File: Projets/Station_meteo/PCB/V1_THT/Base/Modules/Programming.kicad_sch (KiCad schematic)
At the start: 15 parts, among them J13 USB_C_Receptacle_USB2.0_16P, J14 SolderJumper_2_Bridged, J15 SolderJumper_2_Bridged, J16 SolderJumper_2_Bridged, U10 CH340G, U8 USBLC6-2P6, U9 AMS1117-3.3, Y2 12MHz

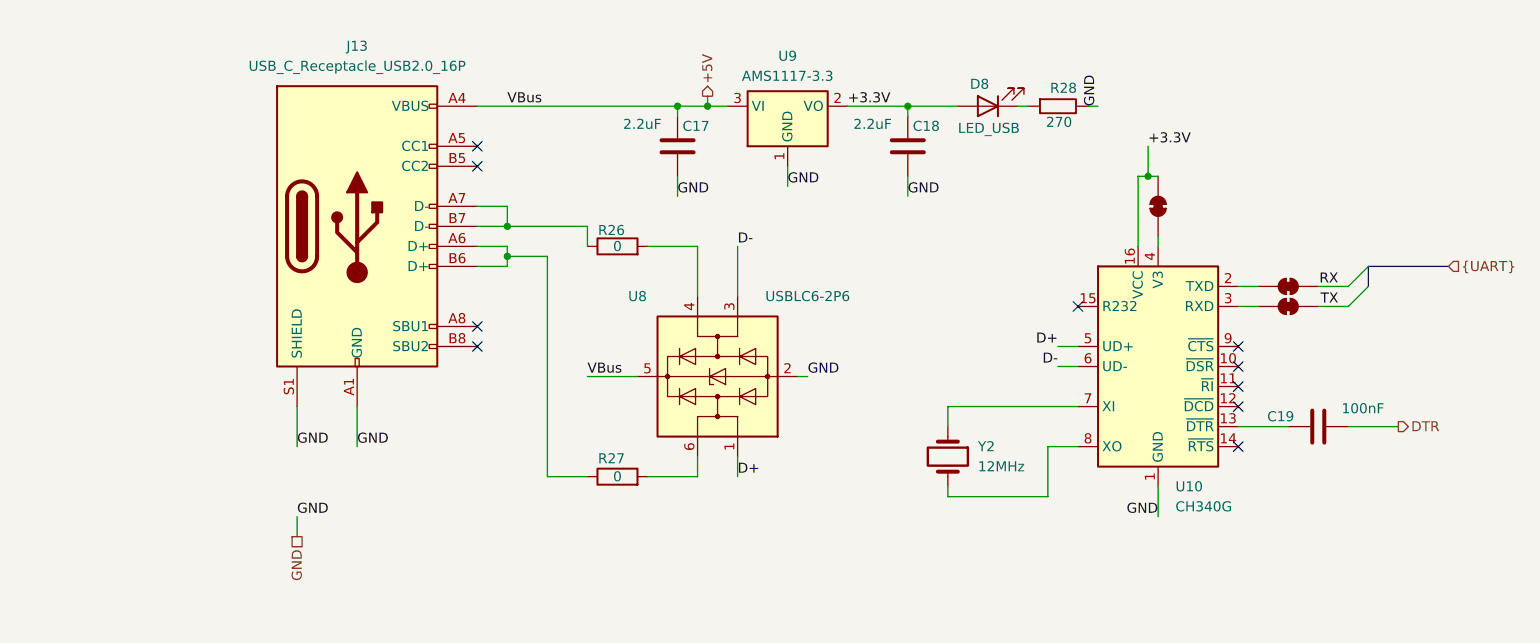
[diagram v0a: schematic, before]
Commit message: Update PCB Base
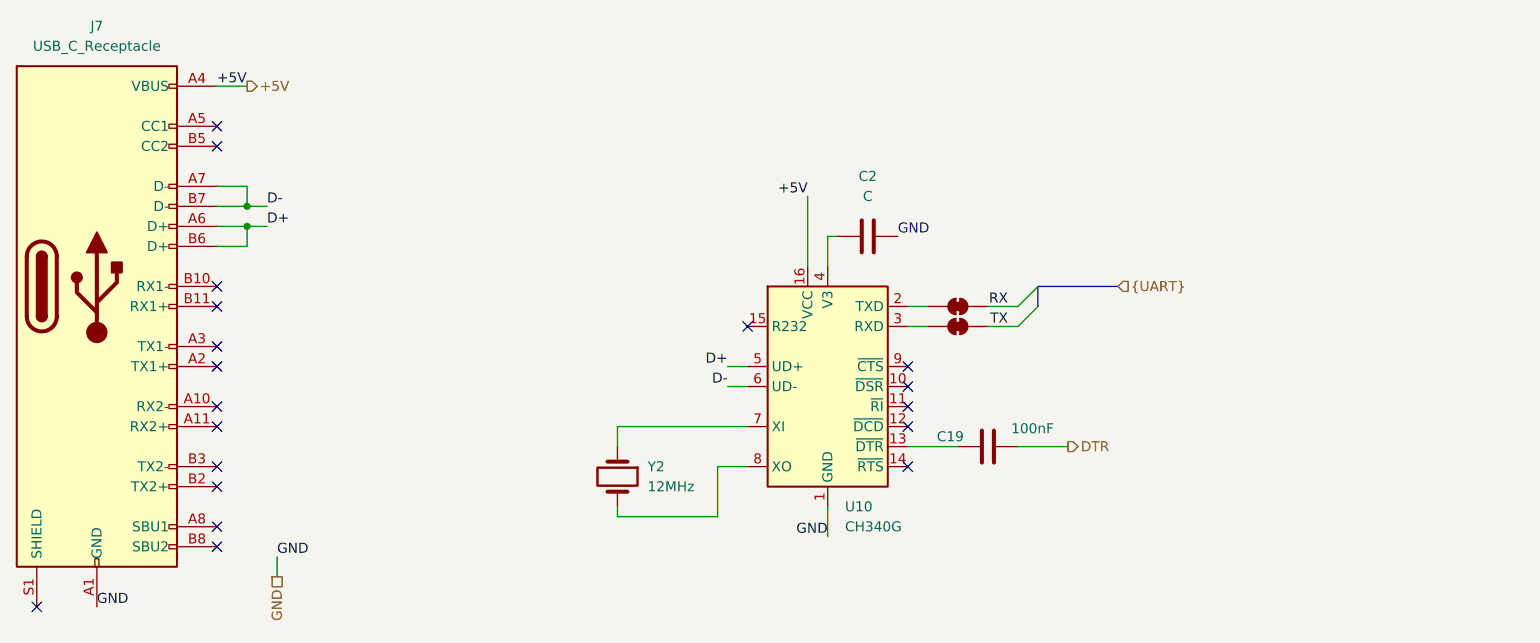
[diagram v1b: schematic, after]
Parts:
- removed C17, C18: 2.2uF, Capacitor_SMD:C_0603_1608Metric, symbol Device:C
- removed D8: LED_USB, LED_SMD:LED_0603_1608Metric, symbol Device:LED
- removed J13: USB_C_Receptacle_USB2.0_16P, Connector_USB:USB_C_Receptacle_GCT_USB4085, symbol Connector:USB_C_Receptacle_USB2.0_16P
- removed J14: SolderJumper_2_Bridged, Jumper:SolderJumper-2_P1.3mm_Bridged_Pad1.0x1.5mm, symbol Jumper:SolderJumper_2_Bridged
- removed R26, R27: 0, Resistor_SMD:R_0603_1608Metric, symbol Device:R
- removed R28: 270, Resistor_SMD:R_0603_1608Metric, symbol PCM_SL_Devices:Resistor_0.5W
- removed U8: USBLC6-2P6, Package_TO_SOT_SMD:SOT-666, symbol Power_Protection:USBLC6-2P6
- removed U9: AMS1117-3.3, Package_TO_SOT_SMD:SOT-223-3_TabPin2, symbol Regulator_Linear:AMS1117-3.3
- added C2: C, symbol Device:C
- added J7: USB_C_Receptacle, CREPP_Connectors_USB:USB_C_Receptacle_GCT_USB4085, symbol CREPP_Connectors_USB_C:USB_C_Receptacle
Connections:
- net +3.3V is gone; now on net +5V: U10.16 (VCC)
- net +5V: now also J7.A4 (VBUS), J7.A9 (VBUS), J7.B4 (VBUS), J7.B9 (VBUS)
- net D+: now also J7.A6 (D+), J7.B6 (D+)
- net D-: now also J7.A7 (D-), J7.B7 (D-)
- net GND: now also C2.2, J7.A1 (GND), J7.A12 (GND), J7.B1 (GND), J7.B12 (GND)
- net at U10.4 (V3): now also C2.1
- no-connect marks 10 -> 19
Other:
- moved on the sheet: C19, U10, Y2
